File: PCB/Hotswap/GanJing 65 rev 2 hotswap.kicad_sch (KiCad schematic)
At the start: 155 parts, among them SW1 EC11_rotary_encoder, U1 Elite-C

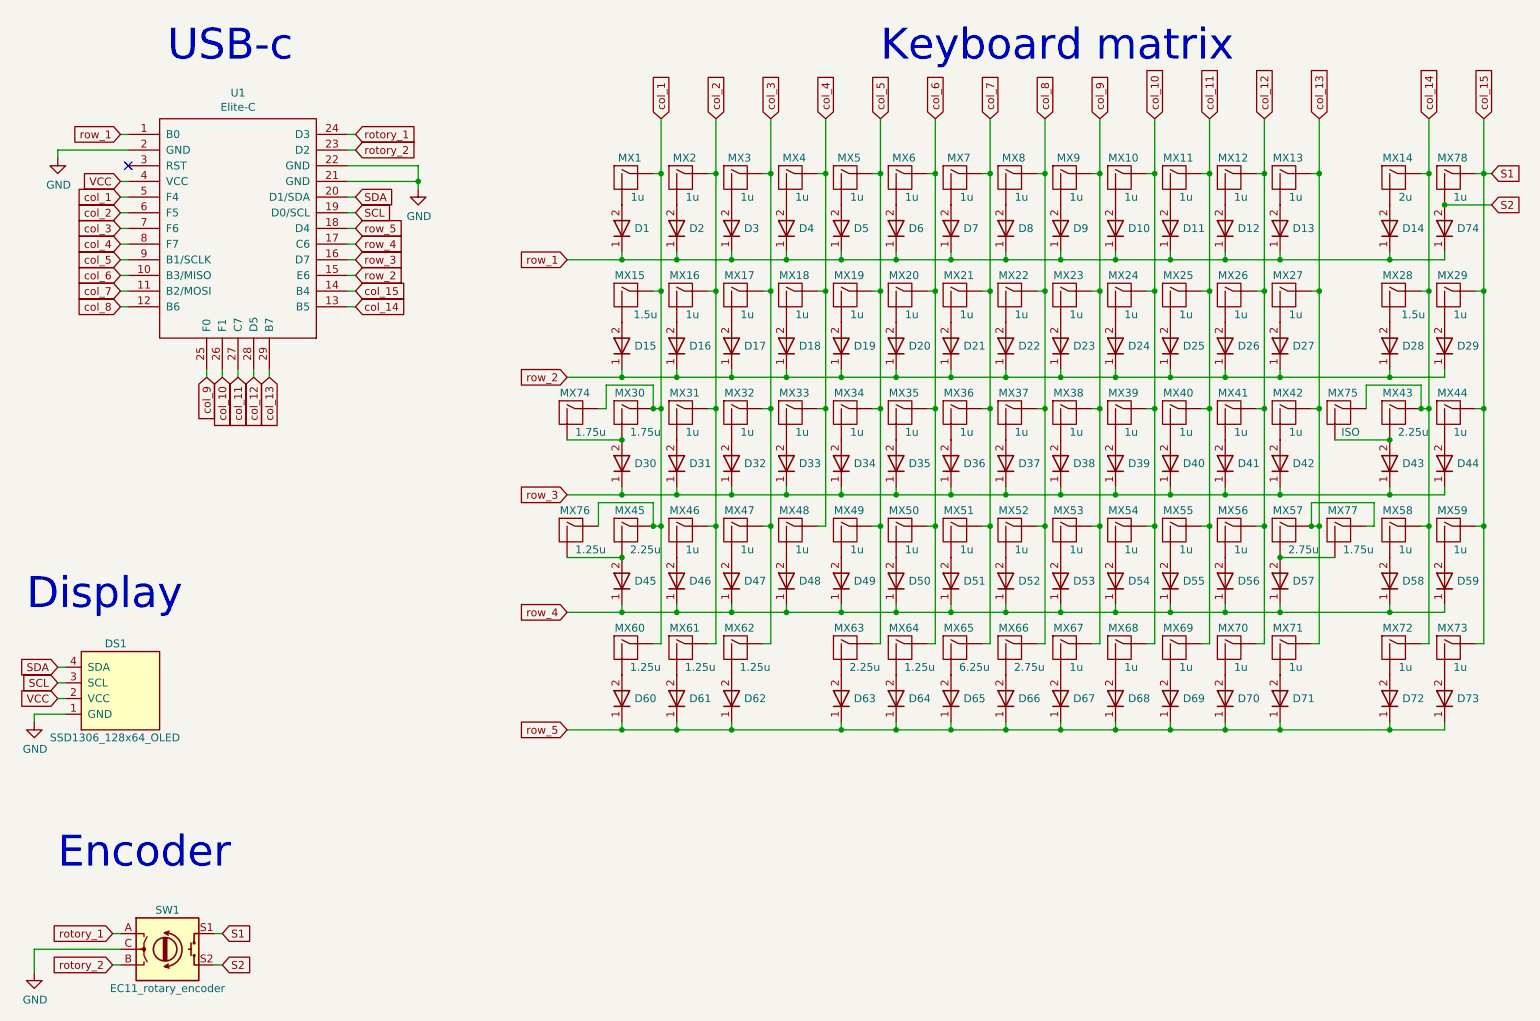
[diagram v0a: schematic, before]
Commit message: Updating soldered version
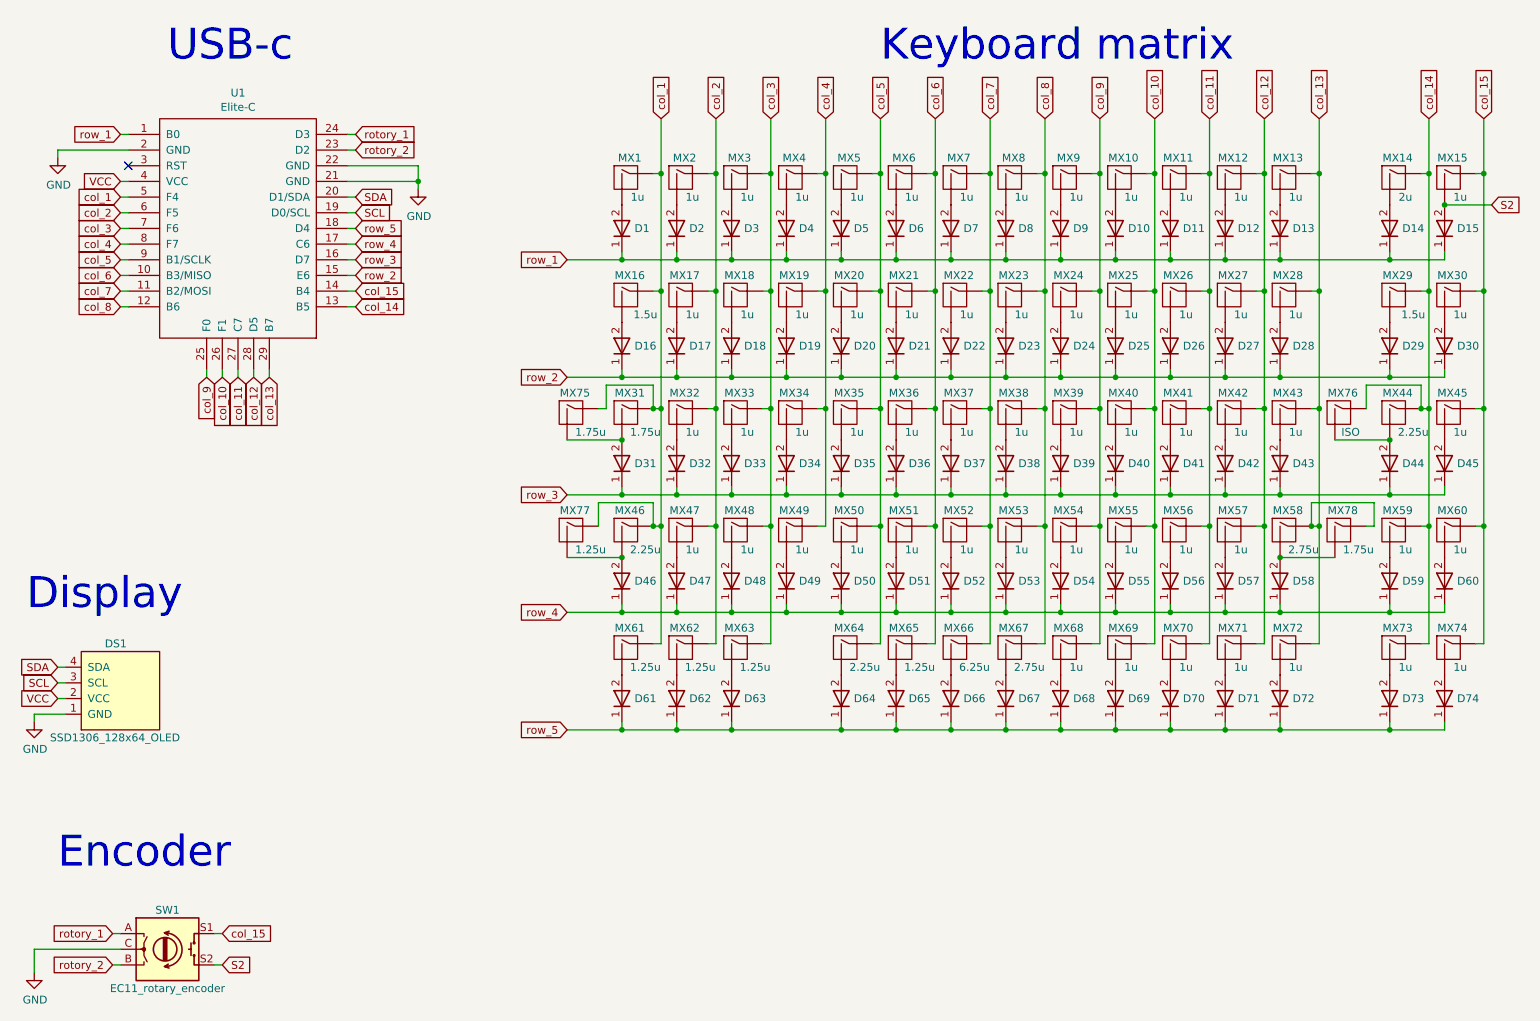
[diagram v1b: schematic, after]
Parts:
- renumbered D74 to D15, D15 to D16, D16 to D17, D17 to D18, D18 to D19, D19 to D20, D20 to D21, D21 to D22, D22 to D23, D23 to D24, D24 to D25, D25 to D26, D26 to D27, D27 to D28, D28 to D29, D29 to D30, D30 to D31, D31 to D32, D32 to D33, D33 to D34, D34 to D35, D35 to D36, D36 to D37, D37 to D38, D38 to D39, D39 to D40, D40 to D41, D41 to D42, D42 to D43, D43 to D44, D44 to D45, D45 to D46, D46 to D47, D47 to D48, D48 to D49, D49 to D50, D50 to D51, D51 to D52, D52 to D53, D53 to D54, D54 to D55, D55 to D56, D56 to D57, D57 to D58, D58 to D59, D59 to D60, D60 to D61, D61 to D62, D62 to D63, D63 to D64, D64 to D65, D65 to D66, D66 to D67, D67 to D68, D68 to D69, D69 to D70, D70 to D71, D71 to D72, D72 to D73, D73 to D74, MX78 to MX15, MX15 to MX16, MX16 to MX17, MX17 to MX18, MX18 to MX19, MX19 to MX20, MX20 to MX21, MX21 to MX22, MX22 to MX23, MX23 to MX24, MX24 to MX25, MX25 to MX26, MX26 to MX27, MX27 to MX28, MX28 to MX29, MX29 to MX30, MX30 to MX31, MX31 to MX32, MX32 to MX33, MX33 to MX34, MX34 to MX35, MX35 to MX36, MX36 to MX37, MX37 to MX38, MX38 to MX39, MX39 to MX40, MX40 to MX41, MX41 to MX42, MX42 to MX43, MX43 to MX44, MX44 to MX45, MX45 to MX46, MX46 to MX47, MX47 to MX48, MX48 to MX49, MX49 to MX50, MX50 to MX51, MX51 to MX52, MX52 to MX53, MX53 to MX54, MX54 to MX55, MX55 to MX56, MX56 to MX57, MX57 to MX58, MX58 to MX59, MX59 to MX60, MX60 to MX61, MX61 to MX62, MX62 to MX63, MX63 to MX64, MX64 to MX65, MX65 to MX66, MX66 to MX67, MX67 to MX68, MX68 to MX69, MX69 to MX70, MX70 to MX71, MX71 to MX72, MX72 to MX73, MX73 to MX74, MX74 to MX75, MX75 to MX76, MX76 to MX77, MX77 to MX78
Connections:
- net S1 renamed col_15
